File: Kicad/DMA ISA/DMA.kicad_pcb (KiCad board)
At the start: 2 copper layers, 132 x 73.9 mm, 19 parts, among them J1 Conn_02x08_Counter_Clockwise, J9 Bus_ISA_8bit, U1 8237, U2 74LS139, U3 74LS04, U4 74LS670, U5 74LS573

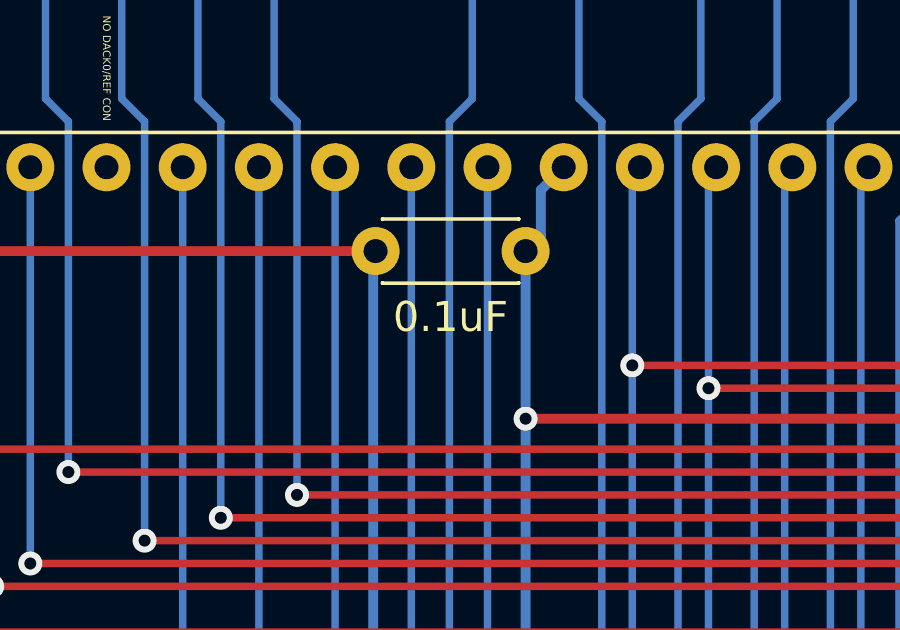
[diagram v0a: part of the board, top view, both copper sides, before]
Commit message: Updated DMA card
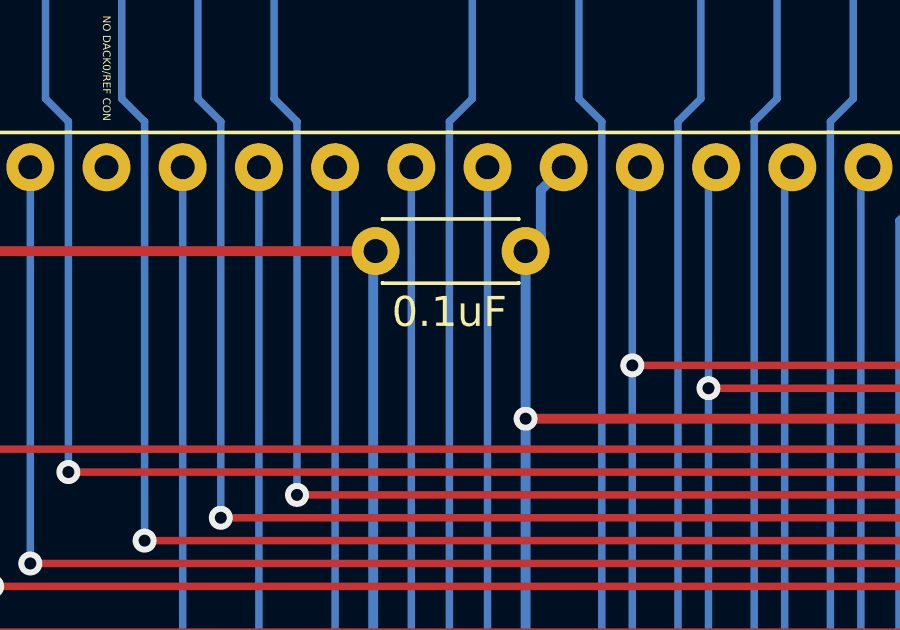
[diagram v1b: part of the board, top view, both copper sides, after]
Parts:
- moved C1 84.4 mm to (77.8, 89.4), turned to 0 degrees
- moved C2 84.4 mm to (158.7, 65.6), turned to 270 degrees
- renumbered R2 to R1, R1 to R2
